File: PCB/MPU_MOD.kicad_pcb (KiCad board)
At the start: 6 copper layers, 47 x 100 mm, 301 parts, among them J501 MEM2090-00-145-00-A_REVA, J701 FTSH-107-01-L-DV-K-A, J801 USB4215-03-A_REVA, J901 73412-0110, U201 STC3115IQT, U202 BQ25606RGER, U203 STPMIC1APQR, U301 STM32MP157FABx, U401 MT41K256M16TW-107_P, U501 EMMC04G-W627-M06U, U502 HSP051-4M10, U503 HSP051-4M10, U701 HSP051-4M10, U702 HSP051-4M10, U801 FUSB302BMPX, U802 HSP051-4M10, U901 LBEE5PK2AE-771, Y601 NX2012SA-32.768K, Y701 ECS-2520MVQ-240

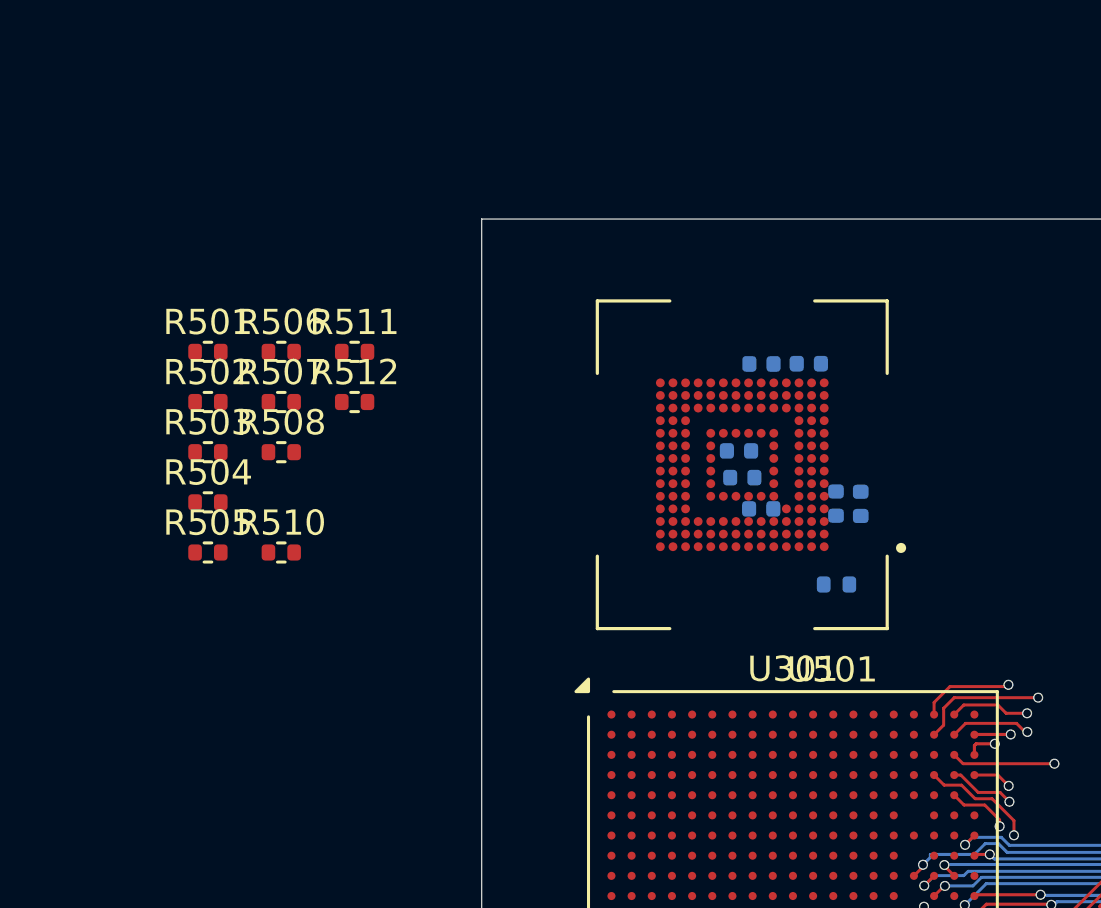
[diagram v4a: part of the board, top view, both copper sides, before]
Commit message: PCD_UPDATE
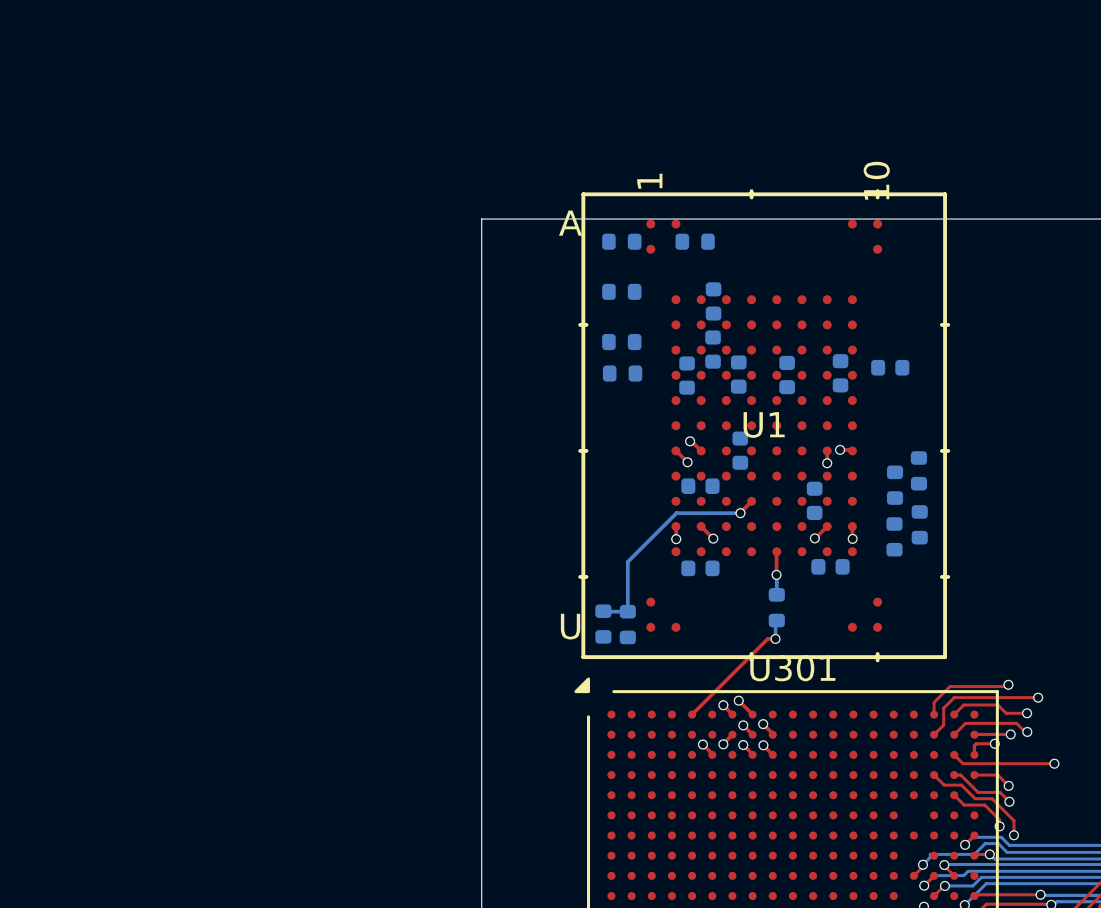
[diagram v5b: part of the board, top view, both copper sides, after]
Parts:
- removed C501: 2.2uF, Capacitor_SMD:C_0402_1005Metric
- removed U501: EMMC04G-W627-M06U, lib:BGA153N50P14X14_1300X1150X100N
- added C509: 1uF, Capacitor_SMD:C_0402_1005Metric, B.Cu at (76.8, 45.4)
- added C510: 100nF, Capacitor_SMD:C_0402_1005Metric, B.Cu at (83.9, 48.0)
- added C511: 100nF, Capacitor_SMD:C_0402_1005Metric, B.Cu at (75.8, 48.4)
- added C512: 100nF, Capacitor_SMD:C_0402_1005Metric, B.Cu at (81.9, 48.3)
- added C513: 100nF, Capacitor_SMD:C_0402_1005Metric, B.Cu at (81.5, 55.9)
- added C514: 100nF, Capacitor_SMD:C_0402_1005Metric, B.Cu at (76.3, 56.0)
- added U1: IS21ES08GA-JQLI-TR, lib:FBGA100_ISI, F.Cu at (78.9, 50.3)
- R501, R502, R503, R504, R505, R506, R507, R508, R510, R511, R512: moved to B.Cu
- moved R505 28.3 mm to (85.0, 54.3), turned to -90 degrees
- moved R503 28.2 mm to (85.0, 52.1), turned to 90 degrees
- moved R502 27.8 mm to (84.0, 54.8), turned to -90 degrees
- moved R504 27.3 mm to (84.0, 52.7), turned to 90 degrees
- moved R501 24.7 mm to (79.4, 57.6), turned to -90 degrees
- moved R511 14.2 mm to (76.1, 43.0), turned to 180 degrees
- moved R506 14.2 mm to (73.2, 43.0), turned to 180 degrees
- moved R507 14.2 mm to (73.2, 45.0), turned to 180 degrees
- moved R508 14.2 mm to (73.2, 47.0), turned to 180 degrees
- moved R512 14.0 mm to (73.5, 58.2), turned to 90 degrees
- moved R510 13.1 mm to (72.5, 58.2), turned to -90 degrees
- moved R509 11.9 mm to (73.2, 48.3), turned to 0 degrees
- moved C502 7.82 mm to (76.8, 47.3), turned to 90 degrees
- moved C507 5.44 mm to (80.9, 53.3), turned to -90 degrees
- moved C504 5.42 mm to (76.3, 52.7), turned to 180 degrees
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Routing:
- net SDMMC2_D7: track 0.00 -> 15.5 mm, vias 0 -> 2
- net SDMMC2_D5: track 0.00 -> 14.0 mm, vias 0 -> 2
- net SDMMC2_D0: track 0.00 -> 13.7 mm, vias 0 -> 2
- net SDMMC2_D2: track 0.00 -> 13.2 mm, vias 0 -> 2
- net SDMMC2_D6: track 0.00 -> 13.1 mm, vias 0 -> 2
- net SDMMC2_D4: track 0.00 -> 9.81 mm, vias 0 -> 2
- net SDMMC2_D3: track 0.00 -> 9.44 mm, vias 0 -> 2
- net SDMMC2_NRST: track 0.00 -> 8.88 mm, vias 0 -> 1
- net SDMMC2_D1: track 0.00 -> 8.72 mm, vias 0 -> 2
- net SDMMC2_CK: track 0.00 -> 5.30 mm, vias 0 -> 1
- net Net-(U1-CLK): track 0.00 -> 1.72 mm, vias 0 -> 1
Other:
- copper layers 6 -> 8
